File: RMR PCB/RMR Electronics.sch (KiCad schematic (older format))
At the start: 6 parts, among them J1 Conn_01x02_Female

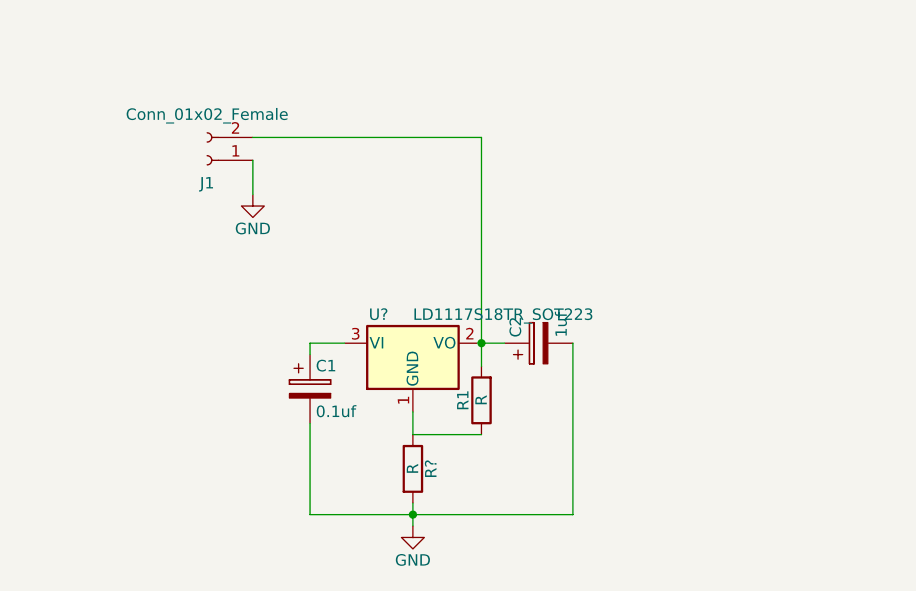
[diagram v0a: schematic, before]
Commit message: V1 of the pcb design
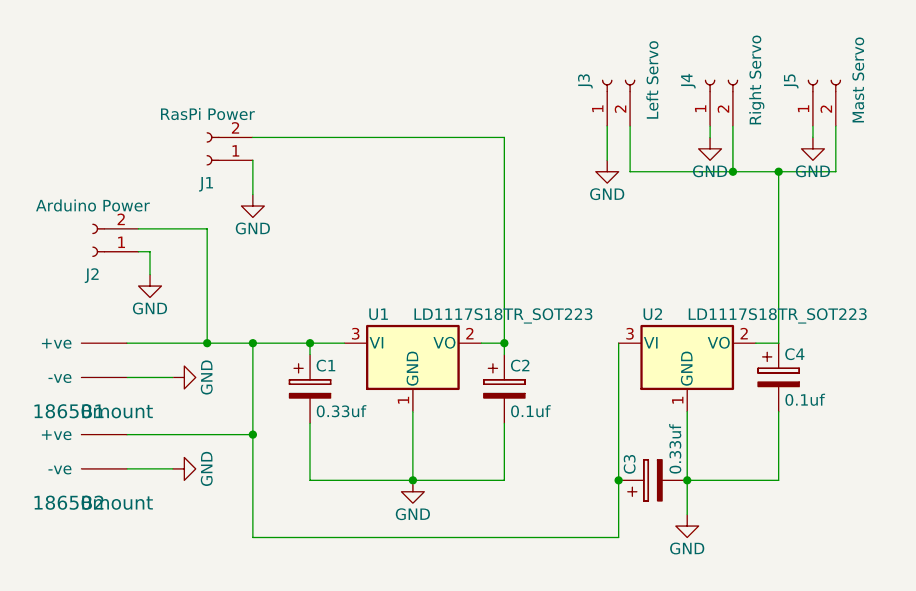
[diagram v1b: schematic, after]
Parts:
- removed R1, R?: R, symbol R
- added B1, B2: 18650mount, symbol 18650mount
- added C3: 0.33uf, symbol CP
- added C4: 0.1uf, symbol CP
- added J2: Arduino Power, symbol Conn_01x02_Female
- added J3: Left Servo, symbol Conn_01x02_Female
- added J4: Right Servo, symbol Conn_01x02_Female
- added J5: Mast Servo, symbol Conn_01x02_Female
- added U2: LD1117S18TR_SOT223, TO_SOT_Packages_SMD:SOT-223-3Lead_TabPin2, symbol LD1117S18TR_SOT223
- C1: value 0.1uf -> 0.33uf
- C2: value 1uf -> 0.1uf
- J1: value Conn_01x02_Female -> RasPi Power
- gave numbers to parts that had none: 1
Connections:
- net GND: now also U1.1 (GND), B1.~ (-ve), B2.~ (-ve), C3.2, C4.2, J2.1 (Pin_1), J3.1 (Pin_1), J4.1 (Pin_1), J5.1 (Pin_1), U2.1 (GND)
- net at C1.1, U1.3 (VI): now also B1.~ (-ve), B2.~ (-ve), C3.1, J2.2 (Pin_2), U2.3 (VI)
- new net: C4.1, J3.2 (Pin_2), J4.2 (Pin_2), J5.2 (Pin_2), U2.2 (VO)
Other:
- moved on the sheet: C2
